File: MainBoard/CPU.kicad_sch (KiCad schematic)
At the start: 2 parts, among them SW1 SW_Push, U2 ESP32-C3-MINI-1

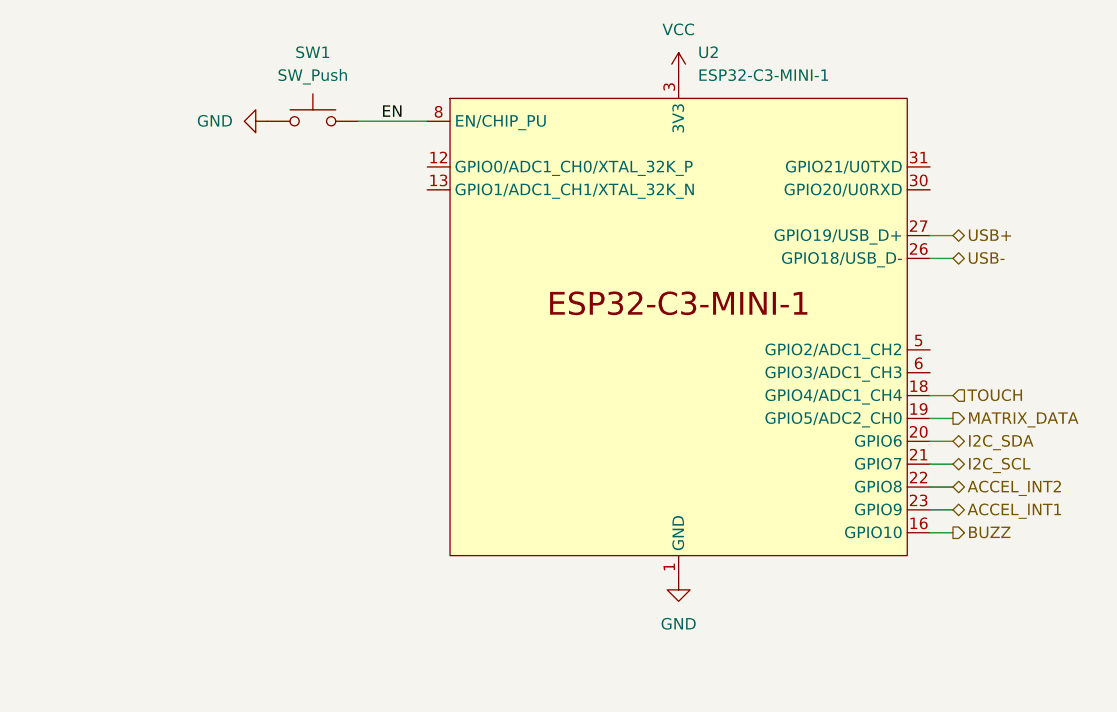
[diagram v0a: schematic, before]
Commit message: change schematic
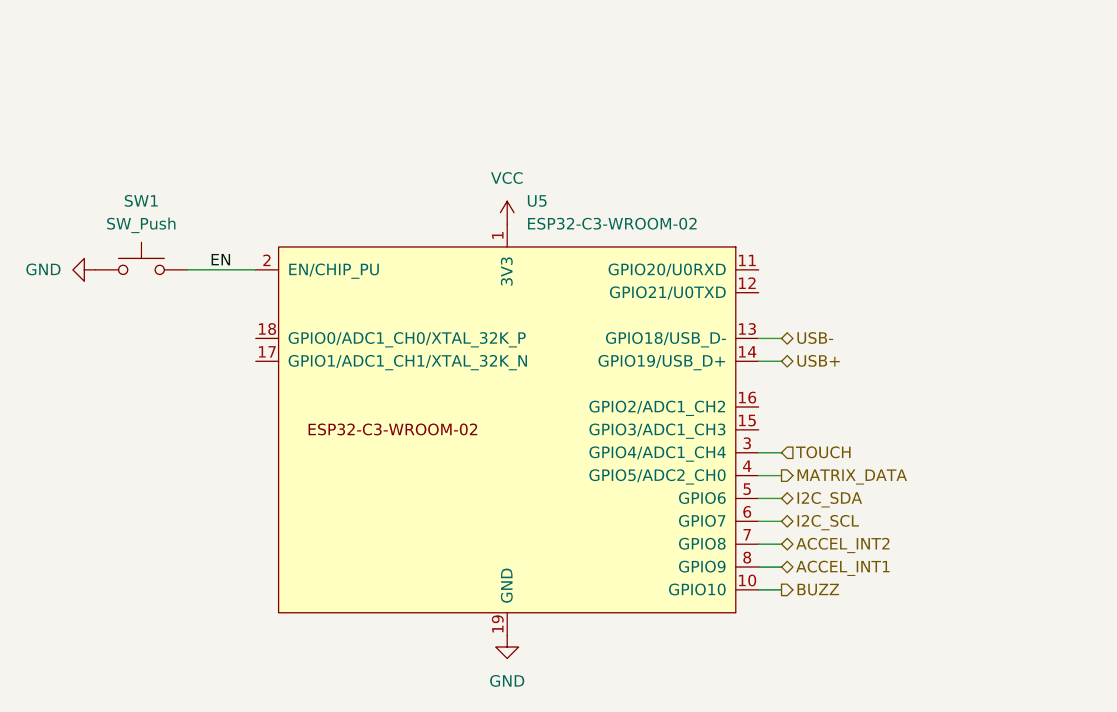
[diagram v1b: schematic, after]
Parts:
- removed U2: ESP32-C3-MINI-1, PCM_Espressif:ESP32-C3-MINI-1, symbol Espressif:ESP32-C3-MINI-1
- added U5: ESP32-C3-WROOM-02, PCM_Espressif:ESP32-C3-WROOM-02, symbol PCM_Espressif:ESP32-C3-WROOM-02
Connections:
- net ACCEL_INT1: now also U5.8 (GPIO9)
- net ACCEL_INT2: now also U5.7 (GPIO8)
- net BUZZ: now also U5.10 (GPIO10)
- net EN: now also U5.2 (EN/CHIP_PU)
- net GND: now also U5.19 (GND), U5.9 (GND)
- net I2C_SCL: now also U5.6 (GPIO7)
- net I2C_SDA: now also U5.5 (GPIO6)
- net MATRIX_DATA: now also U5.4 (GPIO5/ADC2_CH0)
- net TOUCH: now also U5.3 (GPIO4/ADC1_CH4)
- net USB+: now also U5.14 (GPIO19/USB_D+)
- net USB-: now also U5.13 (GPIO18/USB_D-)
- net VCC: now also U5.1 (3V3)
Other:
- moved on the sheet: SW1
